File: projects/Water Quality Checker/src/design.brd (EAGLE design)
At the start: 61 x 107.9 mm, 35 parts, among them Q2 NPN, U1 LM358_SOIC, U2 TPS61073

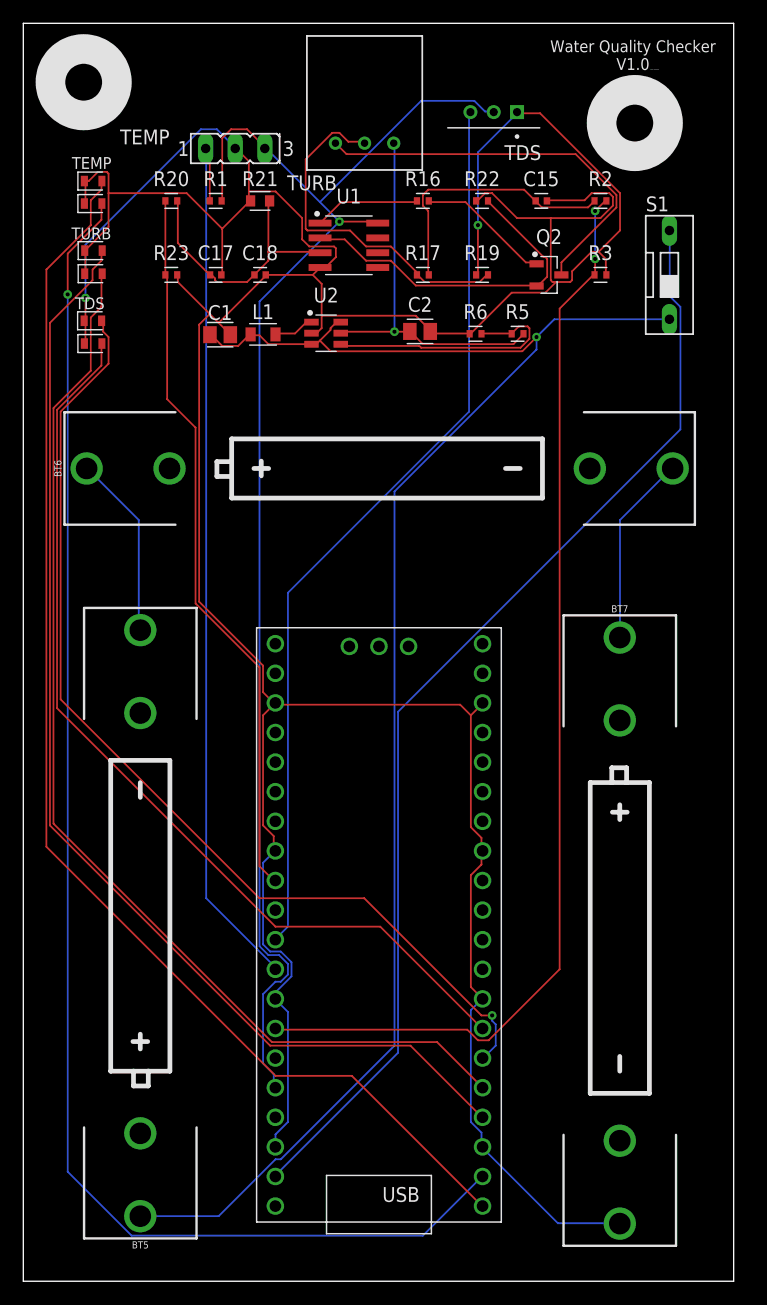
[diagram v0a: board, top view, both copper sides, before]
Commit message: update files
Signed-off-by: Shreyans Jain <shreyans@shreyans.sh>
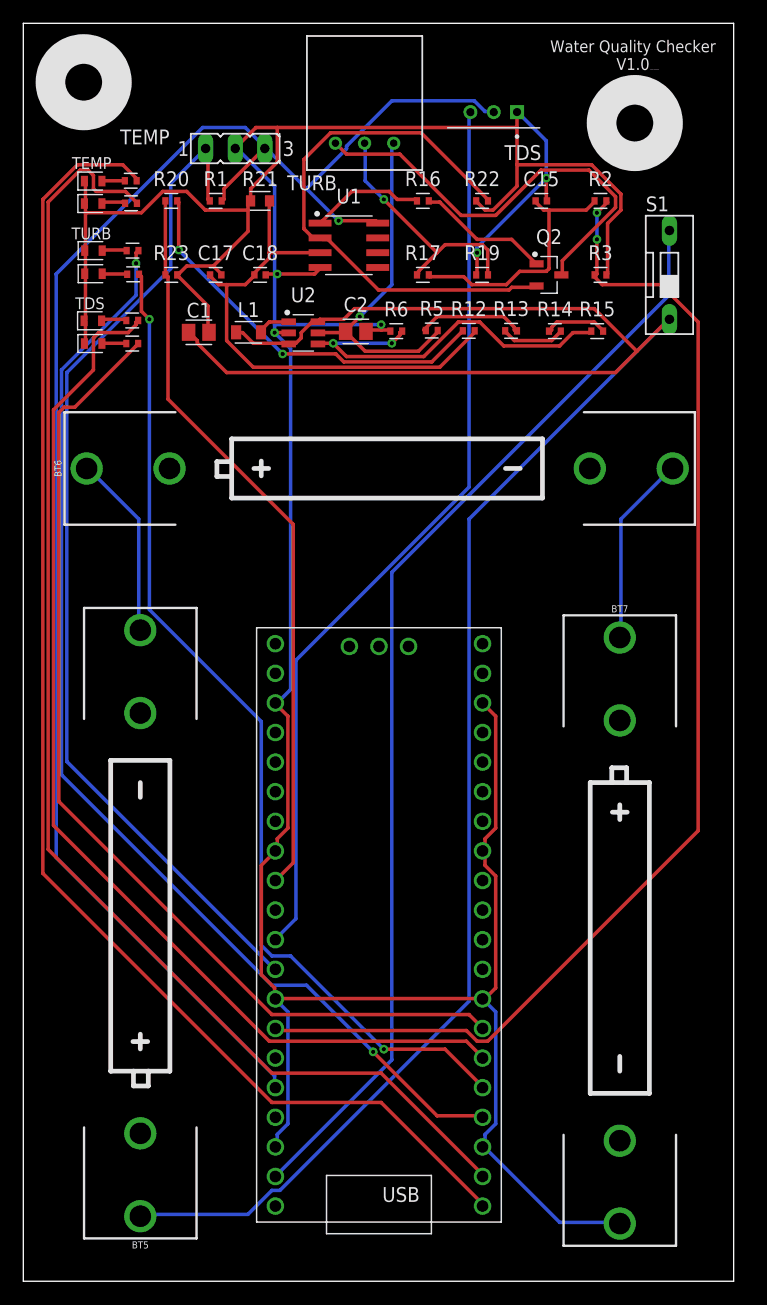
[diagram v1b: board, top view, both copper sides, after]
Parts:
- added R10, R11, R4, R7, R8, R9: 150R, Resistor:RESC1005X40
- added R12: 200R, Resistor:RESC1005X40
- added R13, R14, R15: 200K, Resistor:RESC1005X40
- L1: value 4.7µH -> 10µH
- R20: value 680R -> 470R
- R5: value 1.6M -> 1M
- moved R5 7.37 mm to (4.57, 21.9)
- moved R6 6.81 mm to (1.52, 21.8)
- moved C2 5.51 mm to (-1.94, 21.8)
- moved U2 1.96 mm to (-6.45, 21.7)
- moved C1 1.84 mm to (-15.4, 21.7)
- moved L1 1.26 mm to (-11.2, 21.7)
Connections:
- removed net N$15: R5.1, R6.2, U2.4
- new net N$17: R4.2, U$1.1
- new net N$18: R7.2, U$1.2
- new net N$19: R8.2, U$1.4
- new net N$20: R9.2, U$1.5
- new net N$21: R10.1, TDS_R.A
- new net N$22: R11.2, U$1.7
- new net N$23: R12.1, R20.2
- new net N$24: R13.2, R5.1
- new net N$25: R13.1, R14.2
- new net N$26: R14.1, R15.2
- new net N$27: R15.1, R6.2, U2.4
- net N$10: now also R8.1; no longer U$1.4
- net N$11: now also R9.1; no longer U$1.5
- net N$12: now also R11.1; no longer U$1.7
- net N$13: now also R10.2; no longer TDS_R.A
- net N$45: now also R12.2; no longer R20.2
- net N$8: now also R4.1; no longer U$1.1
- net N$9: now also R7.1; no longer U$1.2
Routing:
- net N$9: track 124.3 -> 2.06 mm, vias 1 -> 0
- net N$17: track 0.00 -> 117.5 mm
- net N$18: track 0.00 -> 115.2 mm
- net N$8: track 109.3 -> 1.97 mm
- net N$10: track 98.7 -> 2.11 mm
- net N$19: track 0.00 -> 96.1 mm, vias 0 -> 2
- net N$11: track 95.1 -> 2.15 mm
- net N$22: track 0.00 -> 87.1 mm
- net N$20: track 0.00 -> 86.0 mm, vias 0 -> 2
- net N$12: track 80.8 -> 2.10 mm
- net VBAT: track 138.5 -> 184.1 mm, vias 1 -> 0
- net N$23: track 0.00 -> 33.7 mm, vias 0 -> 2
- net N$27: track 0.00 -> 33.0 mm, vias 0 -> 2
- net GND: track 341.2 -> 309.9 mm, vias 2 -> 5
- net N$15: track 22.1 -> 0.00 mm
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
